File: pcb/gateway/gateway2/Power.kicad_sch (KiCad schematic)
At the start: 14 parts, among them U3 RT6150AGQW

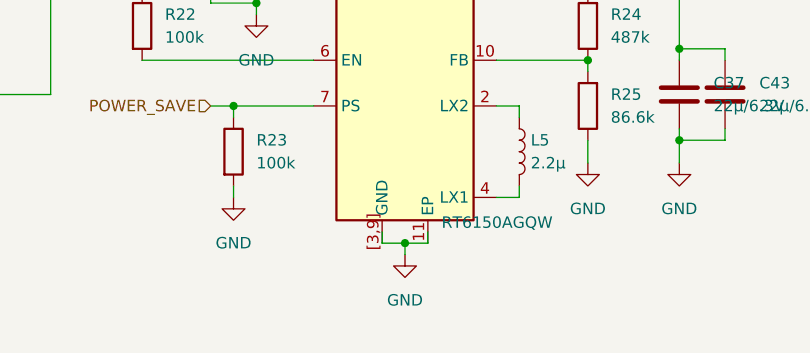
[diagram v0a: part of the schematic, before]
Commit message: Still routing.
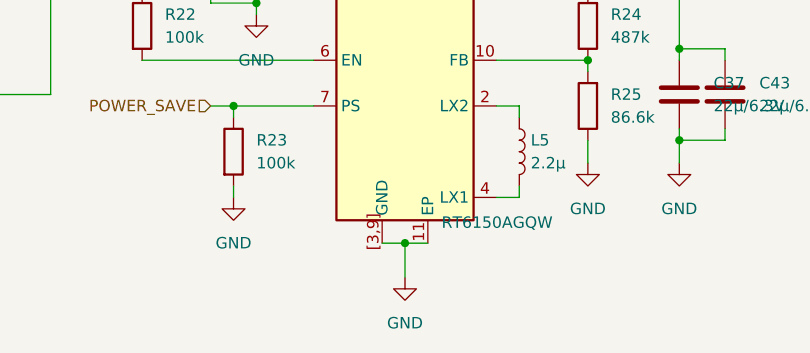
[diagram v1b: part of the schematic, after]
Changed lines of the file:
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@@
+	)
+	(junction
+		(at 190.5 106.68)
+		(diameter 0)
+		(color 0 0 0 0)
 	)
 	(junction
@@
 	)
 	(junction
-		(at 190.5 106.68)
-		(diameter 0)
-		(color 0 0 0 0)
-	)
-	(junction
 		(at 173.99 80.01)
 		(diameter 0)
@@
 	(wire
 		(pts
-			(xy 187.96 105.41) (xy 187.96 106.68)
+			(xy 190.5 106.68) (xy 190.5 110.49)
+		)
+		(stroke
+			(width 0)
+			(type default)
+		)
+	)
+	(wire
+		(pts
+			(xy 107.95 80.01) (xy 107.95 81.28)
+		)
+		(stroke
+			(width 0)
+			(type default)
+		)
+	)
+	(wire
+		(pts
+			(xy 226.06 95.25) (xy 220.98 95.25)
+		)
+		(stroke
+			(width 0)
+			(type default)
+		)
+	)
+	(wire
+		(pts
+			(xy 226.06 86.36) (xy 226.06 85.09)
+		)
+		(stroke
+			(width 0)
+			(type default)
+		)
+	)
+	(wire
+		(pts
+			(xy 168.91 78.74) (xy 168.91 80.01)
+		)
+		(stroke
+			(width 0)
+			(type default)
+		)
+	)
+	(wire
+		(pts
+			(xy 200.66 86.36) (xy 210.82 86.36)
+		)
+		(stroke
+			(width 0)
+			(type default)
+		)
+	)
+	(wire
+		(pts
+			(xy 210.82 95.25) (xy 210.82 97.79)
+		)
+		(stroke
+			(width 0)
+			(type default)
+		)
+	)
+	(wire
+		(pts
+			(xy 107.95 80.01) (xy 113.03 80.01)
 		)
 		(stroke
@@
 	(wire
 		(pts
-			(xy 190.5 106.68) (xy 190.5 107.95)
-		)
-		(stroke
-			(width 0)
-			(type default)
-		)
-	)
-	(wire
-		(pts
-			(xy 107.95 80.01) (xy 107.95 81.28)
-		)
-		(stroke
-			(width 0)
-			(type default)
-		)
-	)
-	(wire
-		(pts
-			(xy 226.06 95.25) (xy 220.98 95.25)
-		)
-		(stroke
-			(width 0)
-			(type default)
-		)
-	)
-	(wire
-		(pts
-			(xy 226.06 86.36) (xy 226.06 85.09)
-		)
-		(stroke
-			(width 0)
-			(type default)
-		)
-	)
-	(wire
-		(pts
-			(xy 168.91 78.74) (xy 168.91 80.01)
-		)
-		(stroke
-			(width 0)
-			(type default)
-		)
-	)
-	(wire
-		(pts
-			(xy 200.66 86.36) (xy 210.82 86.36)
-		)
-		(stroke
-			(width 0)
-			(type default)
-		)
-	)
-	(wire
-		(pts
-			(xy 210.82 95.25) (xy 210.82 97.79)
-		)
-		(stroke
-			(width 0)
-			(type default)
-		)
-	)
-	(wire
-		(pts
-			(xy 107.95 80.01) (xy 113.03 80.01)
-		)
-		(stroke
-			(width 0)
-			(type default)
-		)
-	)
-	(wire
-		(pts
 			(xy 179.07 62.23) (xy 179.07 68.58)
 		)
@@
 	(wire
 		(pts
-			(xy 193.04 105.41) (xy 193.04 106.68)
-		)
-		(stroke
-			(width 0)
-			(type default)
-		)
-	)
-	(wire
-		(pts
 			(xy 179.07 76.2) (xy 180.34 76.2)
 		)
@@
 	(wire
 		(pts
-			(xy 193.04 106.68) (xy 190.5 106.68)
-		)
-		(stroke
-			(width 0)
-			(type default)
-		)
-	)
-	(wire
-		(pts
 			(xy 140.97 66.04) (xy 140.97 68.58)
 		)
@@
 		(pts
 			(xy 140.97 68.58) (xy 168.91 68.58)
+		)
+		(stroke
+			(width 0)
+			(type default)
+		)
+	)
+	(wire
+		(pts
+			(xy 190.5 106.68) (xy 193.04 106.68)
 		)
 		(stroke
@@
 	(symbol
 		(lib_id "power:GND")
-		(at 190.5 107.95 0)
+		(at 190.5 110.49 0)
 		(unit 1)
 		(body_style 1)
@@
 		(fields_autoplaced yes)
 		(property "Reference" "#PWR054"
-			(at 190.5 114.3 0)
+			(at 190.5 116.84 0)
 			(hide yes)
 			(show_name no)
@@
 		)
 		(property "Value" "GND"
-			(at 190.5 113.03 0)
+			(at 190.5 115.57 0)
 			(show_name no)
 			(do_not_autoplace no)
@@
 		)
 		(property "Footprint" ""
-			(at 190.5 107.95 0)
+			(at 190.5 110.49 0)
 			(hide yes)
 			(show_name no)
@@
 		)
 		(property "Datasheet" ""
-			(at 190.5 107.95 0)
+			(at 190.5 110.49 0)
 			(hide yes)
 			(show_name no)
@@
 		)
 		(property "Description" "Power symbol creates a global label with name \"GND\" , ground"
-			(at 190.5 107.95 0)
+			(at 190.5 110.49 0)
 			(hide yes)
 			(show_name no)
